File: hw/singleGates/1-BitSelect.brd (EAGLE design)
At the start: 15 parts, among them Q1 BC817, Q2 BC817, Q3 BC817, Q4 BC817, Q5 BC817, Q6 BC817

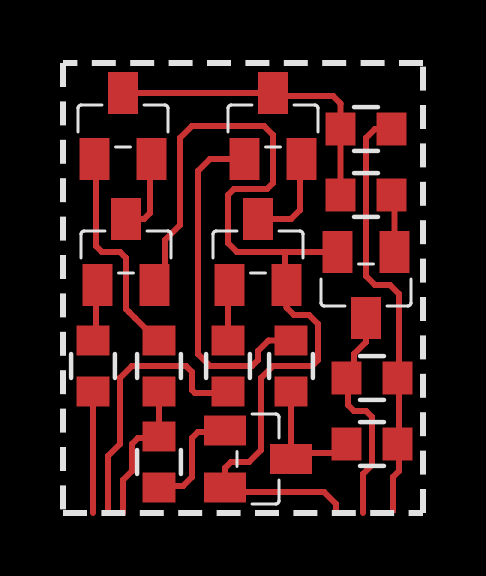
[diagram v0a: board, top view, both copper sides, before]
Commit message: Fixing stuff
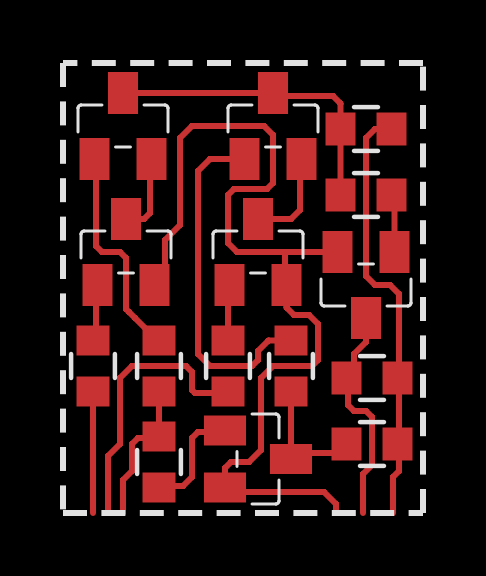
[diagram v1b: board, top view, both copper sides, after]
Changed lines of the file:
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@@
 <?xml version="1.0" encoding="utf-8"?>
 <!DOCTYPE eagle SYSTEM "eagle.dtd">
-<eagle version="7.4.0">
+<eagle version="7.3.0">
 <drawing>
 <settings>
@@
 <wire x1="10.1" y1="12.5" x2="10.4" y2="12.8" width="0.2" layer="1"/>
 <wire x1="10.4" y1="12.8" x2="10.95" y2="12.8" width="0.2" layer="1"/>
-<wire x1="11" y1="0" x2="11" y2="0.8" width="0.2" layer="1" style="shortdash"/>
+<wire x1="11" y1="0" x2="11" y2="0.8" width="0.2" layer="1"/>
 <wire x1="11" y1="0.8" x2="11" y2="1.2" width="0.2" layer="1"/>
 <wire x1="11" y1="1.2" x2="11.2" y2="1.4" width="0.2" layer="1"/>
